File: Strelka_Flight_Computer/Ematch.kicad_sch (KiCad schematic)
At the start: 16 parts, among them Q10 AP2300, Q11 MMBT2222, Q8 AO3401A, Q9 AO3401A, U15 LM321

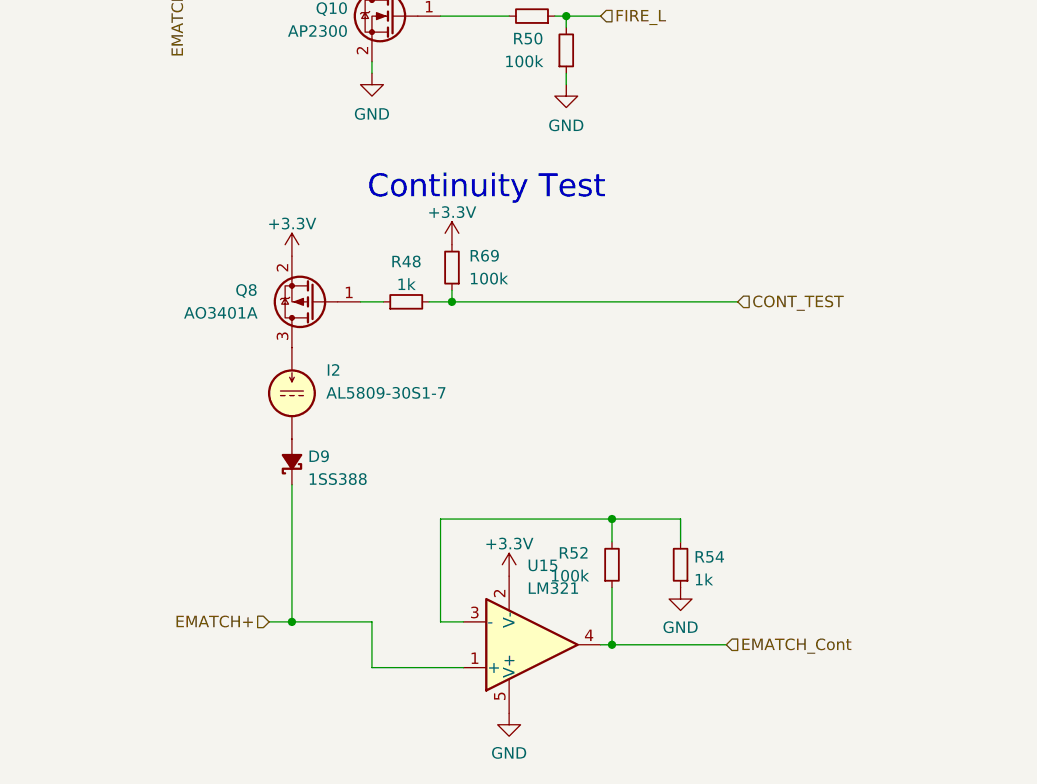
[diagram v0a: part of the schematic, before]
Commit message: Started design for V2
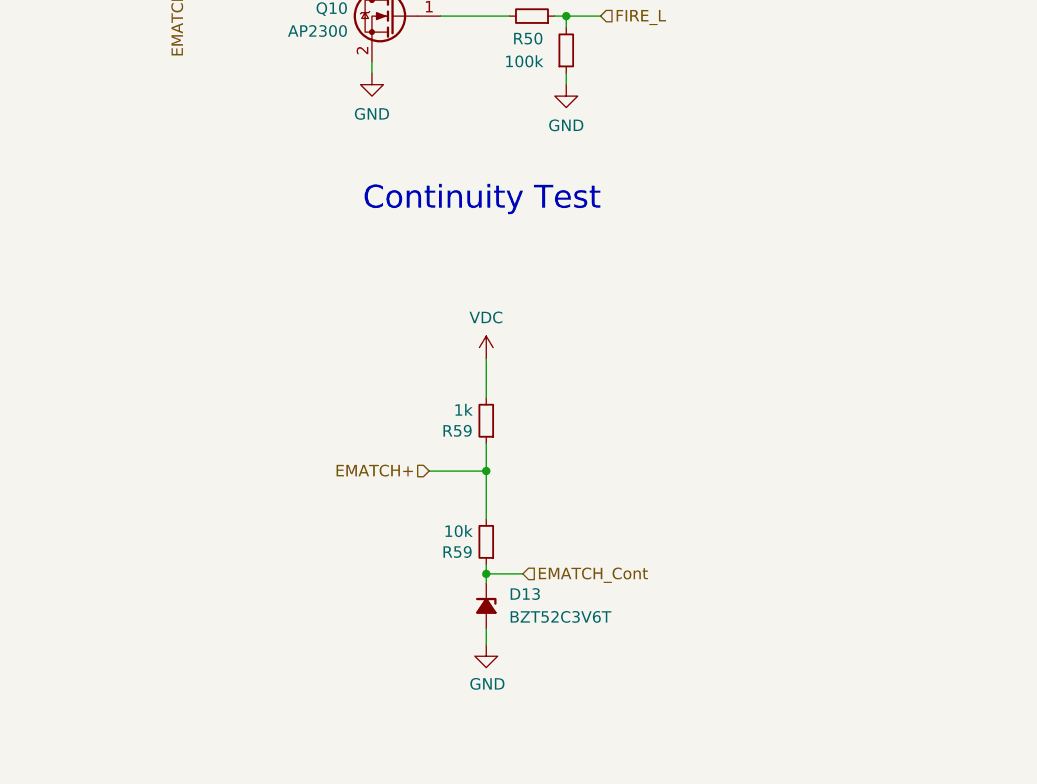
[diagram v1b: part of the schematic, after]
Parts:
- removed D9: 1SS388, Diode_SMD:D_SOD-523, symbol Device:D_Schottky_Small_Filled
- removed I2: AL5809-30S1-7, Diode_SMD:D_SOD-123, symbol Simulation_SPICE:IDC
- removed Q8: AO3401A, Package_TO_SOT_SMD:SOT-23, symbol Transistor_FET:AO3401A
- removed R48, R54: 1k, Resistor_SMD:R_0603_1608Metric, symbol Device:R_Small
- removed R52, R69: 100k, Resistor_SMD:R_0603_1608Metric, symbol Device:R_Small
- removed U15: LM321, Package_TO_SOT_SMD:SOT-23-5, symbol Amplifier_Operational:LM321
- added D13: BZT52C3V6T, Diode_SMD:D_SOD-523, symbol Device:D_Zener_Small_Filled
- added R59: 1k, Resistor_SMD:R_0603_1608Metric, symbol Device:R_Small
- added R59: 10k, Resistor_SMD:R_0603_1608Metric, symbol Device:R_Small
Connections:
- net EMATCH+: now also R59.1, R59.2
- net EMATCH_Cont: now also D13.1 (K), R59.1
- net GND: now also D13.2 (A)
- net VDC: now also R59.2
